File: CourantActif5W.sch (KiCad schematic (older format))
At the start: 2 parts, among them U23 ADC124S021CIMM_NOPB

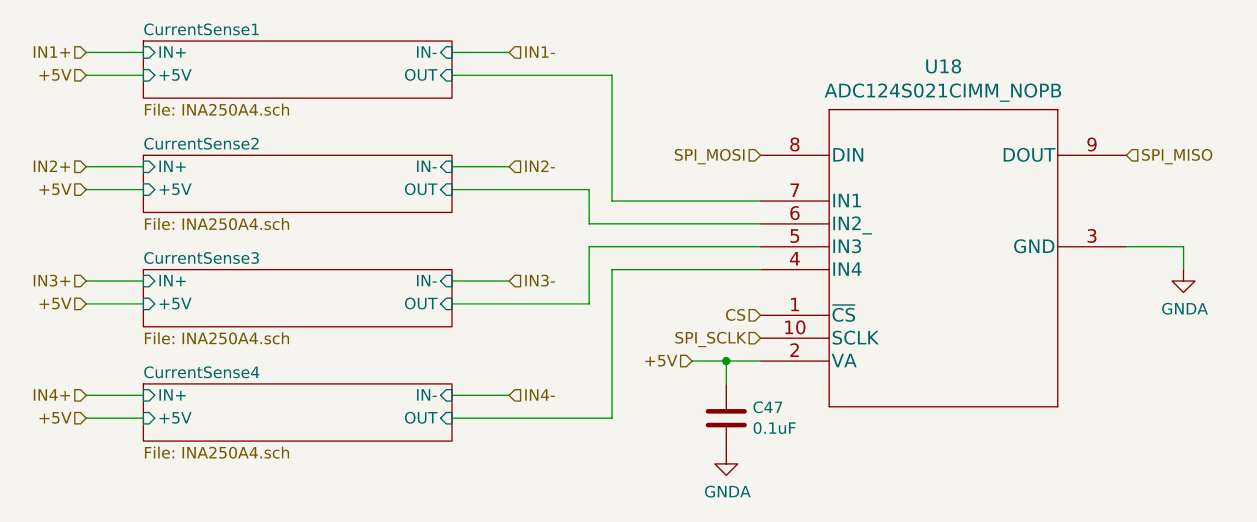
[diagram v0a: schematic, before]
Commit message: routing usb
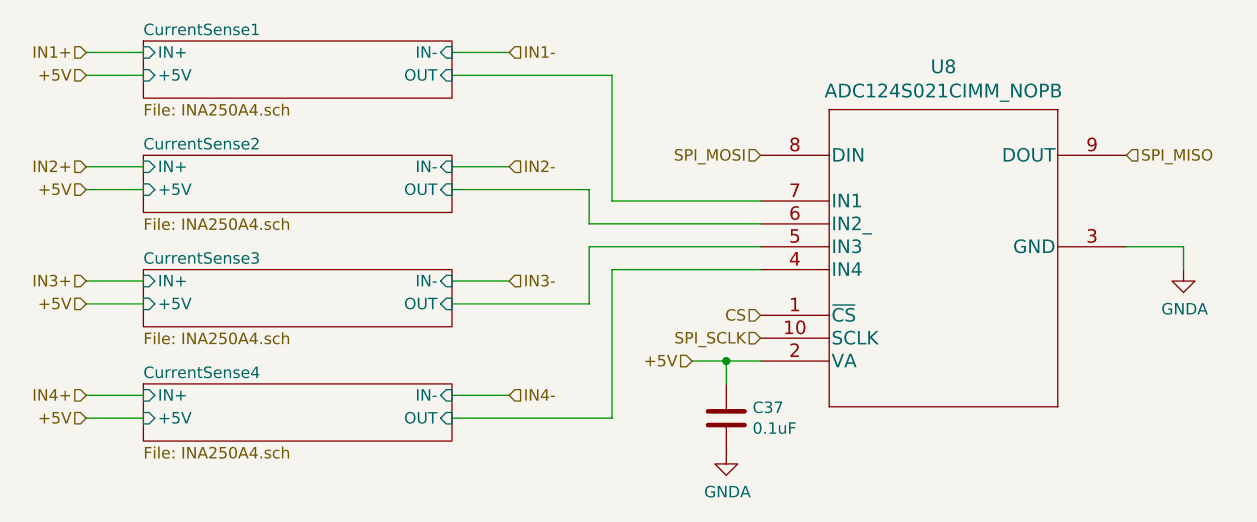
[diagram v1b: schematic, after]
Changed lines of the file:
@@
 $Descr A4 11693 8268
 encoding utf-8
-Sheet 24 80
+Sheet 14 80
 Title ""
 Date "2020-05-19"
@@
 AR Path="/5EEAF65F/5EDDD78D" Ref="U13"  Part="1"
 AR Path="/5EEC30AA/5EDDD78D" Ref="U18"  Part="1"
-F 0 "U18" H 6950 3537 60  0000 C CNN
+F 0 "U8" H 6950 3537 60  0000 C CNN
 F 1 "ADC124S021CIMM_NOPB" H 6950 3431 60  0000 C CNN
 F 2 "Package_SO:VSSOP-10_3x3mm_P0.5mm" H 6950 3390 60  0001 C CNN
@@
 AR Path="/5EEAF65F/5EDF45FB" Ref="C42"  Part="1"
 AR Path="/5EEC30AA/5EDF45FB" Ref="C47"  Part="1"
-F 0 "C47" H 6115 4346 50  0000 L CNN
+F 0 "C37" H 6115 4346 50  0000 L CNN
 F 1 "0.1uF" H 6115 4255 50  0000 L CNN
 F 2 "Capacitor_SMD:C_0402_1005Metric" H 6038 4150 50  0001 C CNN
@@
 AR Path="/5EEC30AA/618421DB" Ref="#PWR090"  Part="1"
 AR Path="/5EC4179E/618421DB" Ref="#PWR0104"  Part="1"
-F 0 "#PWR090" H 8000 3400 50  0001 C CNN
+F 0 "#PWR062" H 8000 3400 50  0001 C CNN
 F 1 "GNDA" H 8005 3477 50  0000 C CNN
 F 2 "" H 8000 3650 50  0001 C CNN
@@
 AR Path="/5EEC30AA/61842231" Ref="#PWR089"  Part="1"
 AR Path="/5EC4179E/61842231" Ref="#PWR0103"  Part="1"
-F 0 "#PWR089" H 6000 4200 50  0001 C CNN
+F 0 "#PWR061" H 6000 4200 50  0001 C CNN
 F 1 "GNDA" H 6005 4277 50  0000 C CNN
 F 2 "" H 6000 4450 50  0001 C CNN

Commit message: Debut routing cannaux passifs
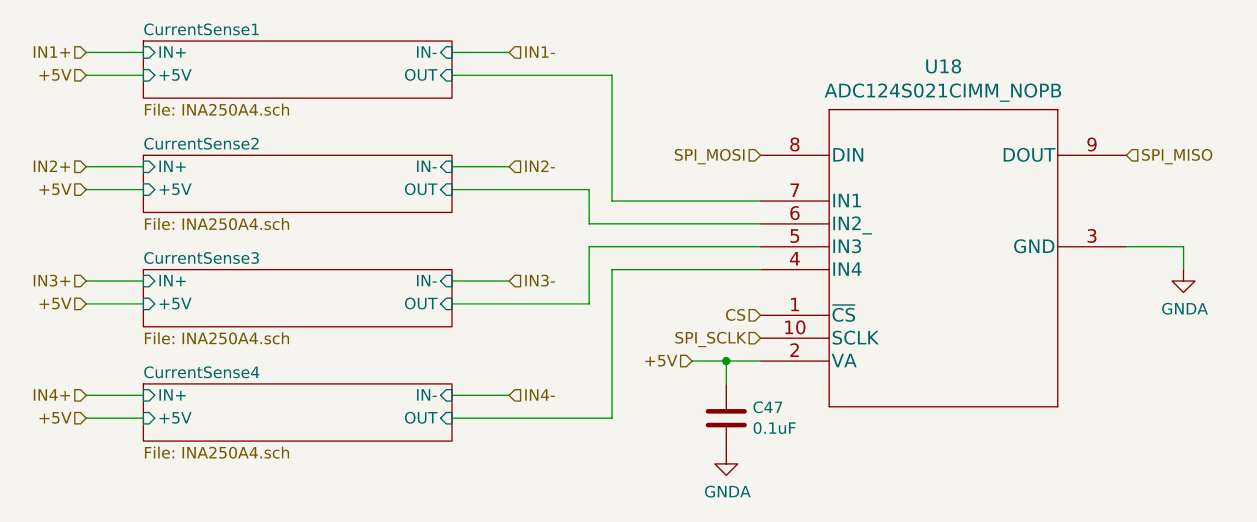
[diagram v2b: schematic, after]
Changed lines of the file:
@@
 $Descr A4 11693 8268
 encoding utf-8
-Sheet 14 80
+Sheet 24 80
 Title ""
 Date "2020-05-19"
@@
 AR Path="/5EEAF65F/5EDDD78D" Ref="U13"  Part="1"
 AR Path="/5EEC30AA/5EDDD78D" Ref="U18"  Part="1"
-F 0 "U8" H 6950 3537 60  0000 C CNN
+F 0 "U18" H 6950 3537 60  0000 C CNN
 F 1 "ADC124S021CIMM_NOPB" H 6950 3431 60  0000 C CNN
 F 2 "Package_SO:VSSOP-10_3x3mm_P0.5mm" H 6950 3390 60  0001 C CNN
@@
 AR Path="/5EEAF65F/5EDF45FB" Ref="C42"  Part="1"
 AR Path="/5EEC30AA/5EDF45FB" Ref="C47"  Part="1"
-F 0 "C37" H 6115 4346 50  0000 L CNN
+F 0 "C47" H 6115 4346 50  0000 L CNN
 F 1 "0.1uF" H 6115 4255 50  0000 L CNN
 F 2 "Capacitor_SMD:C_0402_1005Metric" H 6038 4150 50  0001 C CNN
@@
 AR Path="/5EEC30AA/618421DB" Ref="#PWR090"  Part="1"
 AR Path="/5EC4179E/618421DB" Ref="#PWR0104"  Part="1"
-F 0 "#PWR062" H 8000 3400 50  0001 C CNN
+F 0 "#PWR090" H 8000 3400 50  0001 C CNN
 F 1 "GNDA" H 8005 3477 50  0000 C CNN
 F 2 "" H 8000 3650 50  0001 C CNN
@@
 AR Path="/5EEC30AA/61842231" Ref="#PWR089"  Part="1"
 AR Path="/5EC4179E/61842231" Ref="#PWR0103"  Part="1"
-F 0 "#PWR061" H 6000 4200 50  0001 C CNN
+F 0 "#PWR089" H 6000 4200 50  0001 C CNN
 F 1 "GNDA" H 6005 4277 50  0000 C CNN
 F 2 "" H 6000 4450 50  0001 C CNN
